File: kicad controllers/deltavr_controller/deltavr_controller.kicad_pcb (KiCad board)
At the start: 2 copper layers, 88.8 x 88.8 mm, 52 parts, among them J1 debug, J2 battery pins 3.7v, J3 test 3.3v pins, Q1 IRLZ44N, SW1 SW_Push, SW2 SW_Push, SW3 SW_Push, U10 ADS1115IDGS, U2 nice_nano, U3 SS49E, U4 SS49E, U5 LSM6DSVTR, U6 HT7333, U7 HT7333, U8 HT7333, U9 HT7333

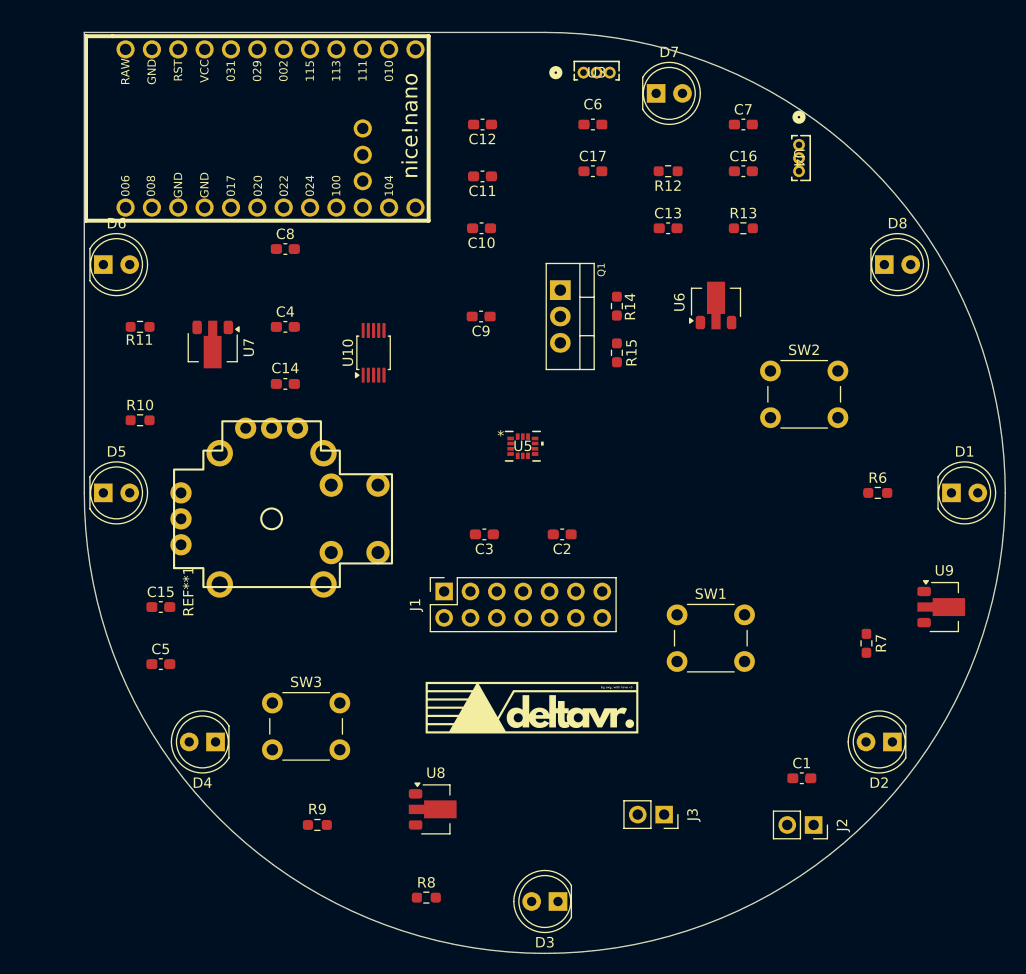
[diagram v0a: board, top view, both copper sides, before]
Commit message: controllers are FUVCKING DONNE AYYYAYYYY
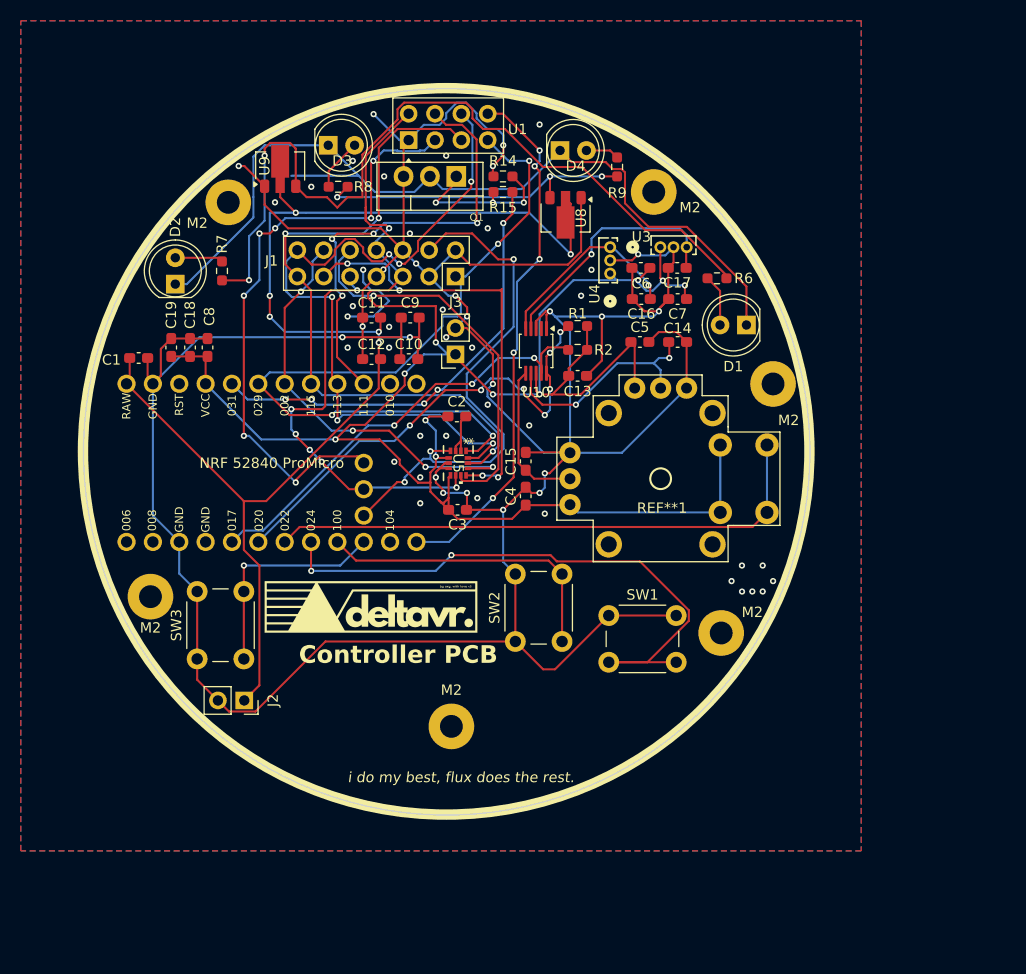
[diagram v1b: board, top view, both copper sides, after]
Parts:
- removed D5, D6, D7, D8: 850nm, LED_THT:LED_D5.0mm_IRGrey
- removed R10, R11, R12, R13: 15Ω, Resistor_SMD:R_0603_1608Metric_Pad0.98x0.95mm_HandSolder
- removed U6, U7: HT7333, Package_TO_SOT_SMD:SOT-89-3
- added C18: 10uF, Capacitor_SMD:C_0603_1608Metric_Pad1.08x0.95mm_HandSolder, F.Cu at (120.3, 75.5)
- added C19: 100nF, Capacitor_SMD:C_0603_1608Metric_Pad1.08x0.95mm_HandSolder, F.Cu at (118.5, 75.5)
- added M2: MountingHole_2.2mm_M2_Pad, MountingHole:MountingHole_2.2mm_M2_Pad, F.Cu at (176.5, 79.0)
- added M2: MountingHole_2.2mm_M2_Pad, MountingHole:MountingHole_2.2mm_M2_Pad, F.Cu at (124.0, 61.5)
- added M2: MountingHole_2.2mm_M2_Pad, MountingHole:MountingHole_2.2mm_M2_Pad, F.Cu at (171.5, 103.0)
- added M2: MountingHole_2.2mm_M2_Pad, MountingHole:MountingHole_2.2mm_M2_Pad, F.Cu at (165.0, 60.5)
- added M2: MountingHole_2.2mm_M2_Pad, MountingHole:MountingHole_2.2mm_M2_Pad, F.Cu at (116.5, 99.5)
- added M2: MountingHole_2.2mm_M2_Pad, MountingHole:MountingHole_2.2mm_M2_Pad, F.Cu at (145.5, 112.0)
- added R1: 4.7kΩ, Resistor_SMD:R_0603_1608Metric_Pad0.98x0.95mm_HandSolder, F.Cu at (157.7, 73.4)
- added R2: 4.7kΩ, Resistor_SMD:R_0603_1608Metric_Pad0.98x0.95mm_HandSolder, F.Cu at (157.7, 75.7)
- added U1: NRF24L01_Breakout, RF_Module:nRF24L01_Breakout, F.Cu at (141.4, 55.5)
- moved D2 82.0 mm to (118.9, 69.4), turned to 90 degrees
- moved U9 76.8 mm to (129.0, 58.0), turned to 90 degrees
- moved D3 76.2 mm to (133.6, 56.0), turned to 0 degrees
- moved C1 75.7 mm to (115.4, 76.5), turned to 180 degrees
- moved R7 71.7 mm to (123.4, 68.1), turned to 90 degrees
- moved R9 69.7 mm to (161.5, 58.1), turned to -90 degrees
- moved R8 69.0 mm to (134.6, 60.0), turned to 180 degrees
- moved D4 66.0 mm to (156.0, 56.5), turned to 0 degrees
- moved U8 58.4 mm to (156.5, 63.0), turned to -90 degrees
- moved J2 56.2 mm to (125.5, 109.5)
- moved C5 55.6 mm to (163.7, 75.0)
- moved J3 48.7 mm to (145.9, 76.1), turned to 180 degrees
- moved C14 38.0 mm to (167.3, 75.0)
- moved C15 37.9 mm to (152.7, 86.5), turned to 90 degrees
- moved REF**1 37.7 mm to (165.7, 88.1)
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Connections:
- net /sensor1 renamed /out1
- net /sensor2 renamed /out2
- C2 pad 2: /3.3v -> /2 - SDX
- C3 pad 1: /3.3v -> /2 - SDX
- C4 pad 2: /3.3v -> /2 - SDX
- C5 pad 2: /3.3v -> /2 - SDX
- U2 pad 12: unconnected-(U2-P1.06-Pad12) -> /8 - IRQ
- U2 pad 15: unconnected-(U2-P1.11-Pad15) -> /4 - CSN
- U2 pad 33: unconnected-(U2-P1.07-Pad33) -> /3 - CE
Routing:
- net /2 - SDX: track 0.00 -> 366.7 mm, vias 0 -> 53
- net /3.3v: track 0.00 -> 206.3 mm, vias 0 -> 12
- net /3.7v(f): track 0.00 -> 132.1 mm, vias 0 -> 7
- net /drain: track 0.00 -> 85.9 mm
- net /l-v1: track 0.00 -> 80.2 mm, vias 0 -> 2
- net /1 - SDO/SAO: track 0.00 -> 74.3 mm, vias 0 -> 4
- net /14 - SDA: track 0.00 -> 72.2 mm, vias 0 -> 6
- net /13 - SCL: track 0.00 -> 65.9 mm, vias 0 -> 3
- net /f1: track 0.00 -> 58.9 mm, vias 0 -> 2
- net /3 - CE: track 0.00 -> 58.9 mm, vias 0 -> 7
- net /joy-btn-gpio: track 0.00 -> 54.2 mm, vias 0 -> 2
- net /8 - IRQ: track 0.00 -> 51.3 mm, vias 0 -> 5
- net /4 - INT1: track 0.00 -> 50.8 mm, vias 0 -> 3
- net /ADC SCL: track 0.00 -> 45.9 mm, vias 0 -> 7
- net /led array mosfet: track 0.00 -> 43.6 mm, vias 0 -> 5
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- added copper zone on B.Cu, net /2 - SDX
- added copper zone on F.Cu, net /2 - SDX
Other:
- board size 88.8 x 88.8 mm -> 70 x 70 mm
- board text added: "'m a pcb..."
- board text added: "-ruan mei"
- board text added: "Controller PCB"
- board text added: "Made with love by [oxy.]"
- board text added: "do not lick the pcb. (okay maybe a little)"
- board text added: "i do my best, flux does the rest."
- board text added: "{dblquote}thanks for choosing to use deltavr. you are appreciated.{dblquote}"
- board text removed: "Controller PCB (R)"
- board text removed: "deltavr."
